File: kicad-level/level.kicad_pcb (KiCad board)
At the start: 2 copper layers, 62.9 x 27.4 mm, 6 parts, among them J1 Conn_01x01_Pin, J2 Conn_01x08_Pin, J3 Conn_01x01_Pin, U1 ULN2803A_C845537

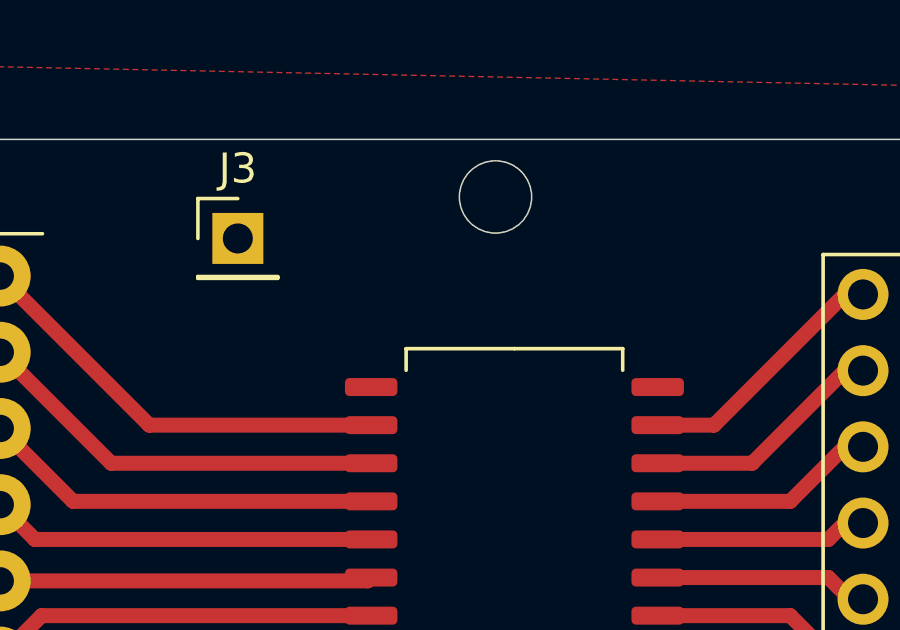
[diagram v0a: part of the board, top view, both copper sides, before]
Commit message: Revert "erreur pcb, com a la masse"
This reverts commit de789b6cb290ad22ceee4c73f03ad83cfbf3b982.
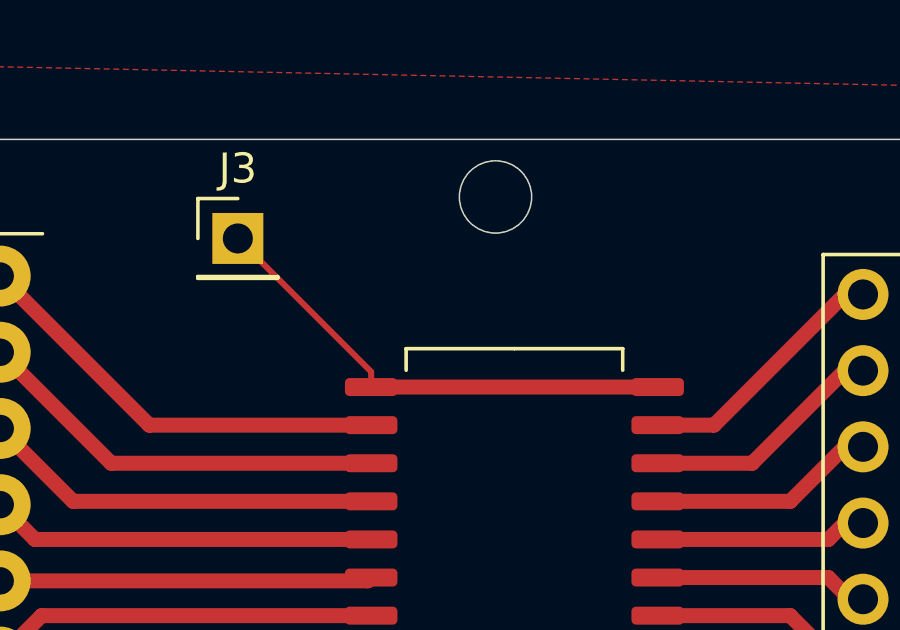
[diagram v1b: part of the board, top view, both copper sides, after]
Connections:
- U1 pad 10: unconnected-(U1-COM-Pad10) -> GND
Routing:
- net GND: track 0.00 -> 16.3 mm
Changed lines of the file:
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@@
 	(net 25 "Net-(J2-Pin_8)")
 	(net 26 "GND")
-	(net 27 "unconnected-(U1-COM-Pad10)")
 	(footprint "Connector_PinHeader_2.54mm:PinHeader_1x08_P2.54mm_Vertical"
 		(layer "F.Cu")
@@
 			(layers "F.Cu" "F.Mask" "F.Paste")
 			(roundrect_rratio 0.25)
-			(net 27 "unconnected-(U1-COM-Pad10)")
+			(net 26 "GND")
 			(pinfunction "COM")
 			(pintype "passive")
@@
 		(net 25)
 	)
+	(segment
+		(start 173.355 92.837)
+		(end 173.355 92.329)
+		(width 0.2)
+		(layer "F.Cu")
+		(net 26)
+	)
+	(segment
+		(start 182.905 92.837)
+		(end 173.355 92.837)
+		(width 0.5)
+		(layer "F.Cu")
+		(net 26)
+	)
+	(segment
+		(start 173.355 92.329)
+		(end 168.91 87.884)
+		(width 0.2)
+		(layer "F.Cu")
+		(net 26)
+	)
 	(zone
